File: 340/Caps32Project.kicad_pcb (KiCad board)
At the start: 2 copper layers, 32 x 20 mm, 37 parts, among them J1 Ph 2.0, J2 Sh 1.0, J4 Sh 2.0, P1 USB_C_Plug_USB2.0, Q1 AO3401A, Q2 MBT3904DW1, SW1 Reset, SW2 Boot, U1 MPU-6050, U2 MAX17048G_T10, U4 MCP73831-2-OT, U5 AP2112K-3.3, U6 ESP32-WROOM-32D

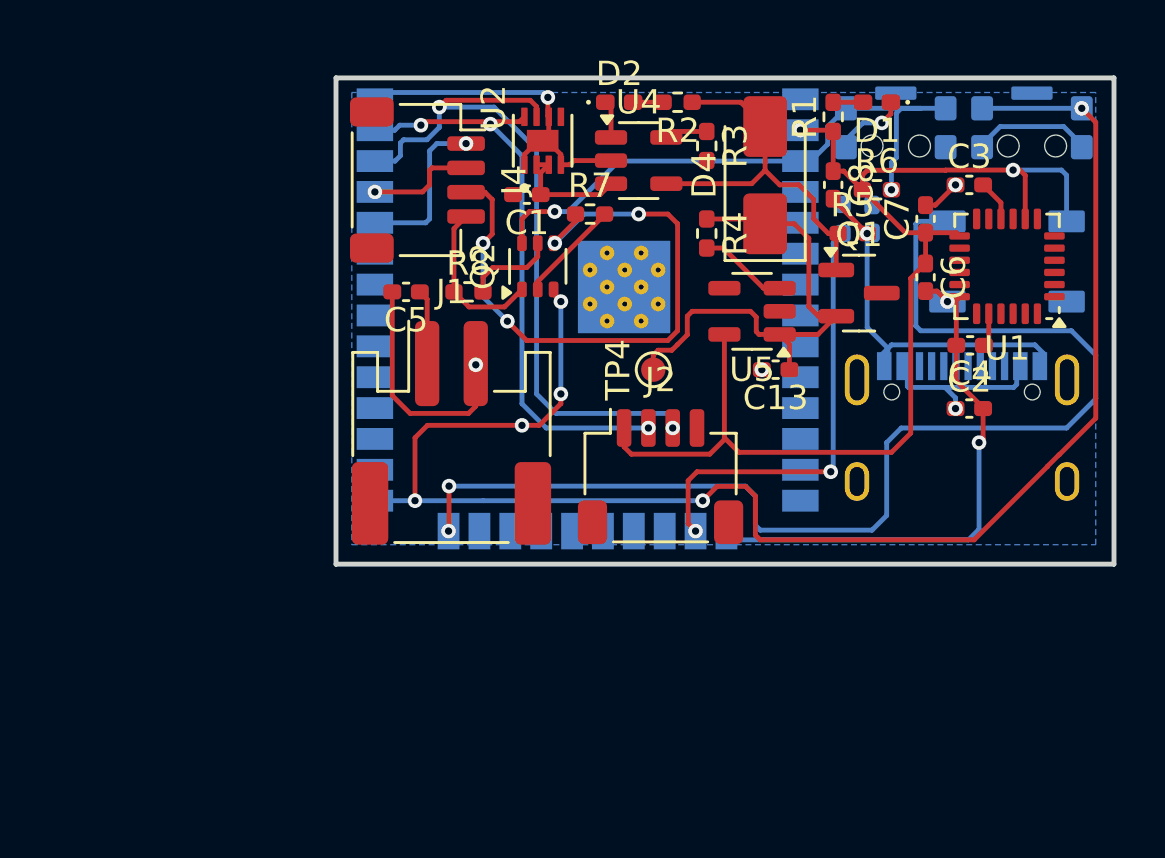
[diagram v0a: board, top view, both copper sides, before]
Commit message: Sync from 340 to main/340
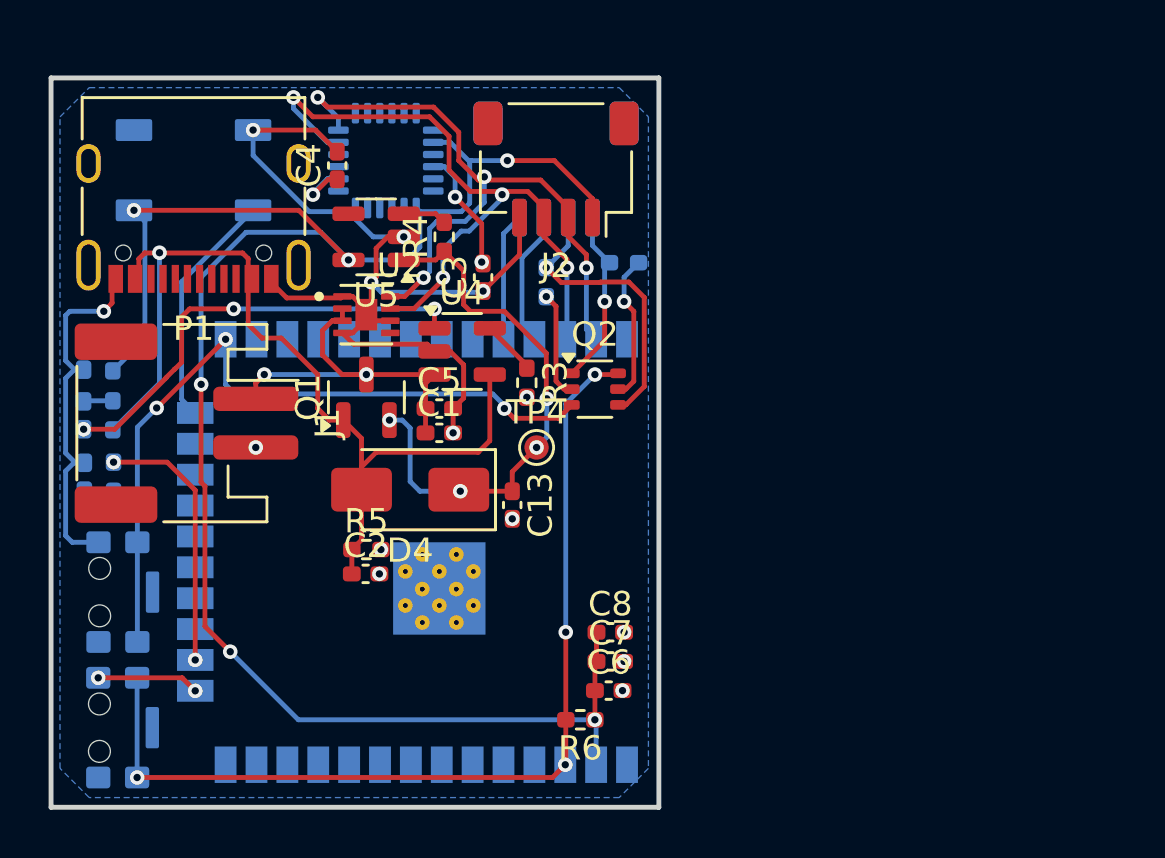
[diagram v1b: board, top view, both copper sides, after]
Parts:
- D1, D2, J4, R1, R2, R7, R8, U1: moved to B.Cu
- P1: moved to F.Cu
- moved SW1 42.2 mm to (16.6, 46.5), turned to 90 degrees
- moved SW2 40.4 mm to (16.6, 52.1), turned to 90 degrees
- moved D1 34.3 mm to (15.2, 36.8), turned to 90 degrees
- moved D5 34.1 mm to (15.2, 41.8), turned to -90 degrees
- moved D3 33.7 mm to (19.7, 29.2), turned to 0 degrees
- moved P1 33.4 mm to (19.7, 30.0)
- moved R9 31.8 mm to (16.4, 41.8), turned to -90 degrees
- moved R1 31.2 mm to (16.4, 36.9)
- moved C4 27.1 mm to (25.6, 29.0), turned to 90 degrees
- moved R2 26.6 mm to (16.4, 39.3), turned to 90 degrees
- moved U1 25.9 mm to (27.6, 28.8), turned to -90 degrees
- moved C2 25.7 mm to (26.8, 45.8)
- moved D2 25.5 mm to (15.2, 39.3), turned to 90 degrees
- moved R6 25.0 mm to (35.6, 51.8), turned to 180 degrees
- moved R5 23.9 mm to (26.8, 44.8)
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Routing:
- net RGB_DI: track 49.1 -> 9.78 mm, vias 2 -> 0
- net 0: track 64.9 -> 30.9 mm, vias 6 -> 3
- net +3V3: track 49.1 -> 78.9 mm, vias 2 -> 6
- net Net-(D2-K): track 1.55 -> 18.4 mm, vias 0 -> 3
- net VBUS: track 23.2 -> 38.9 mm
- net CHIP_PU: track 25.1 -> 39.5 mm, vias 2 -> 4
- net DTR: track 26.0 -> 12.0 mm, vias 4 -> 1
- net GND: track 72.2 -> 61.2 mm, vias 8 -> 16
- net LED: track 18.2 -> 10.8 mm
- net +BATT: track 8.02 -> 15.3 mm, vias 0 -> 2
- net SDA: track 24.1 -> 28.1 mm, vias 3 -> 4
- net Net-(U1-REGOUT): track 1.70 -> 5.02 mm, vias 0 -> 2
- net Net-(Q2B-B2): track 3.75 -> 6.07 mm, vias 0 -> 1
- net Net-(U5-EN): track 3.68 -> 1.81 mm
- net Net-(D4-K): track 20.6 -> 22.5 mm, vias 0 -> 4
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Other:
- board size 32 x 20 mm -> 25 x 30 mm
